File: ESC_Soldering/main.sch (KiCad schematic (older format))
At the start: 15 parts, among them P1 CONN_02X03, P2 CONN_01X03, P3 CONN_01X03, P4 CONN_01X02, P5 CONN_01X10, P6 CONN_01X10, P7 CONN_01X10, U1 PCA9698, U2 ADS7828, U7 Littlebee, U8 Littlebee

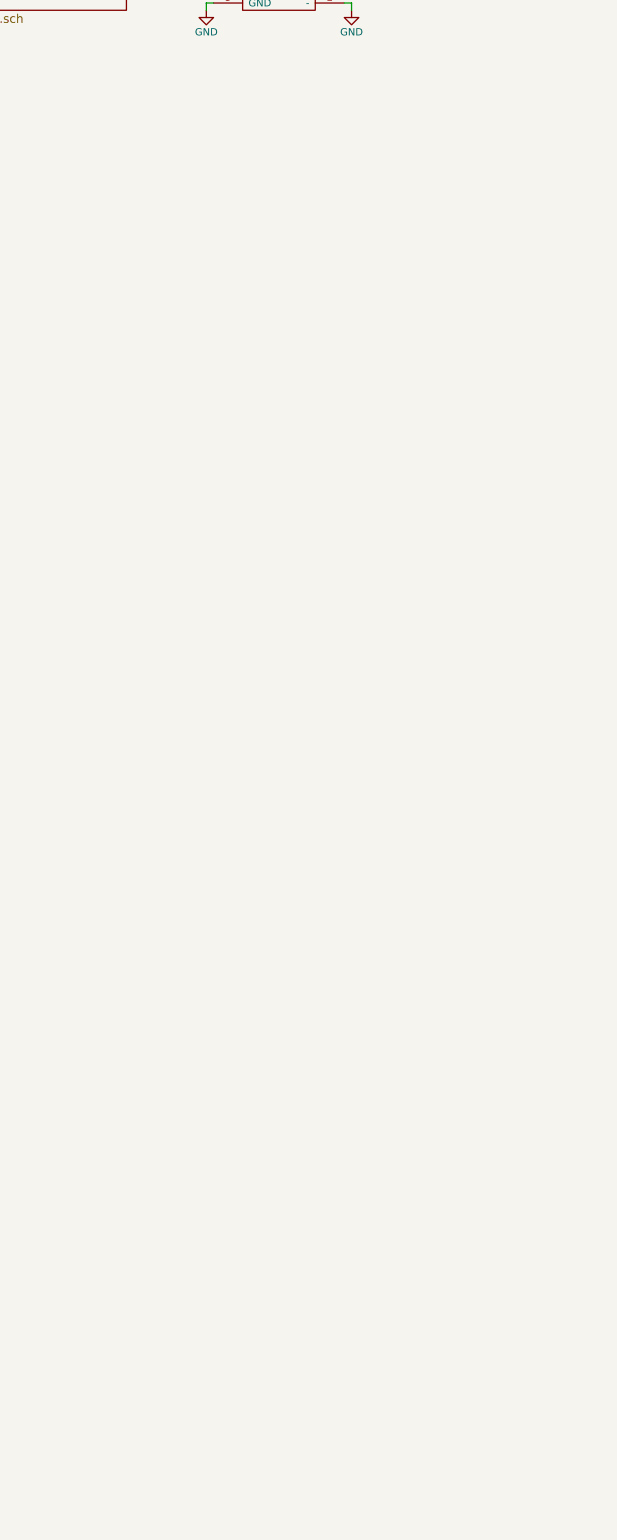
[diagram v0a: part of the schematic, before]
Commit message: test
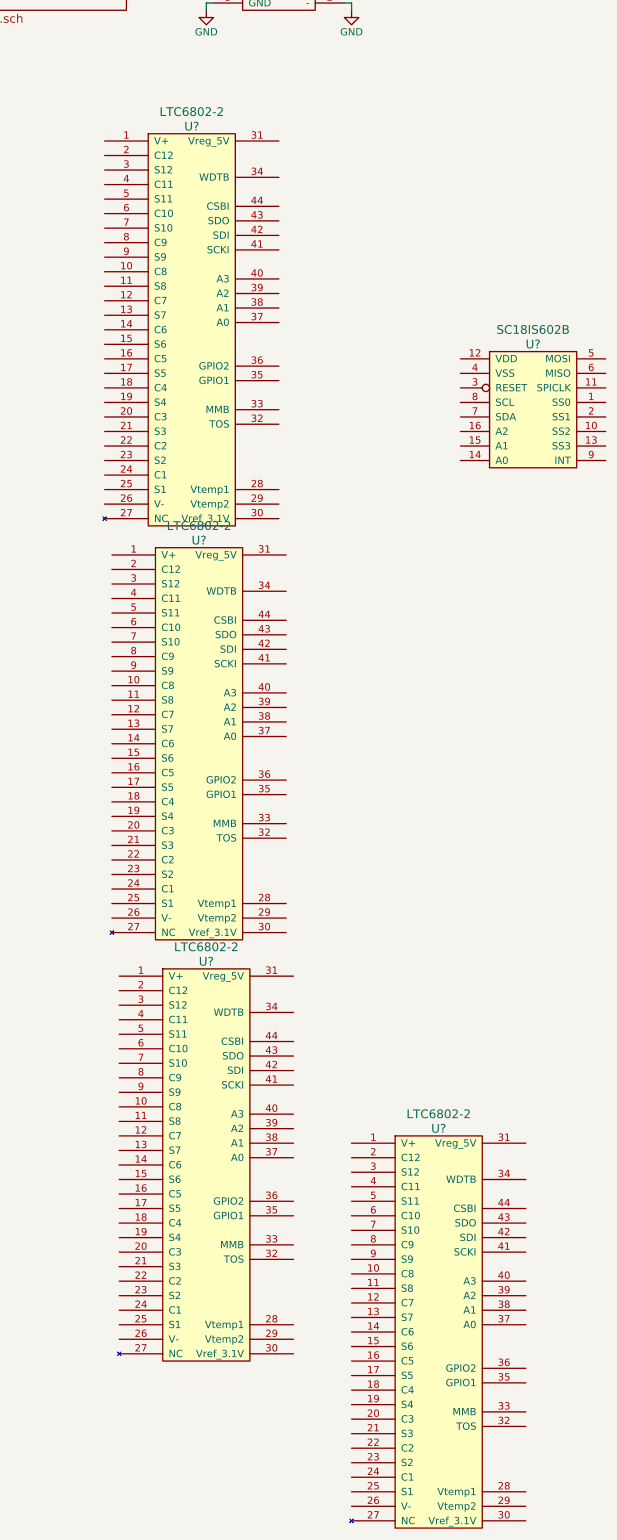
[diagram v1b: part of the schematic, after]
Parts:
- added U? (x4): LTC6802-2, symbol LTC6802-2
- added U?: SC18IS602B, symbol SC18IS602B
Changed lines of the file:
@@
 Text Label 10100 3350 2    60   ~ 0
 Enable_2
+$Comp
+L LTC6802-2 U?
+U 1 1 5854091D
+P 12200 5600
+F 0 "U?" H 12200 6750 60  0000 C CNN
+F 1 "LTC6802-2" H 12200 6850 60  0000 C CNN
+F 2 "" H 11850 5600 60  0000 C CNN
+F 3 "http://cds.linear.com/docs/en/datasheet/68022fa.pdf" H 12200 7200 60  0001 C CNN
+	1    12200 5600
+	1    0    0    -1
+$EndComp
+$Comp
+L SC18IS602B U?
+U 1 1 585409D8
+P 14550 6500
+F 0 "U?" H 14550 7050 60  0000 C CNN
+F 1 "SC18IS602B" H 14550 7150 60  0000 C CNN
+F 2 "" H 14550 6250 60  0001 C CNN
+F 3 "http://www.nxp.com/documents/data_sheet/SC18IS602B.pdf" H 14550 7250 60  0001 C CNN
+	1    14550 6500
+	1    0    0    -1
+$EndComp
+$Comp
+L LTC6802-2 U?
+U 1 1 58540B70
+P 12250 8450
+F 0 "U?" H 12250 9600 60  0000 C CNN
+F 1 "LTC6802-2" H 12250 9700 60  0000 C CNN
+F 2 "" H 11900 8450 60  0000 C CNN
+F 3 "http://cds.linear.com/docs/en/datasheet/68022fa.pdf" H 12250 10050 60  0001 C CNN
+	1    12250 8450
+	1    0    0    -1
+$EndComp
+$Comp
+L LTC6802-2 U?
+U 1 1 58540C42
+P 12300 11350
+F 0 "U?" H 12300 12500 60  0000 C CNN
+F 1 "LTC6802-2" H 12300 12600 60  0000 C CNN
+F 2 "" H 11950 11350 60  0000 C CNN
+F 3 "http://cds.linear.com/docs/en/datasheet/68022fa.pdf" H 12300 12950 60  0001 C CNN
+	1    12300 11350
+	1    0    0    -1
+$EndComp
+$Comp
+L LTC6802-2 U?
+U 1 1 58540D7D
+P 13900 12500
+F 0 "U?" H 13900 13650 60  0000 C CNN
+F 1 "LTC6802-2" H 13900 13750 60  0000 C CNN
+F 2 "" H 13550 12500 60  0000 C CNN
+F 3 "http://cds.linear.com/docs/en/datasheet/68022fa.pdf" H 13900 14100 60  0001 C CNN
+	1    13900 12500
+	1    0    0    -1
+$EndComp
 $EndSCHEMATC
